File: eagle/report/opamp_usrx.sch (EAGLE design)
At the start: 11 parts, among them IC1 LM324N

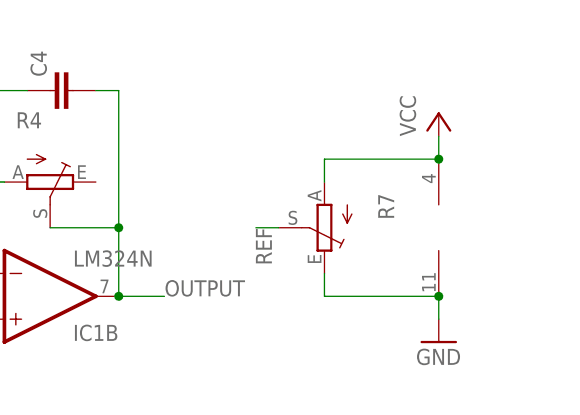
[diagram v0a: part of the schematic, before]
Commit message: Continued design and implementation.
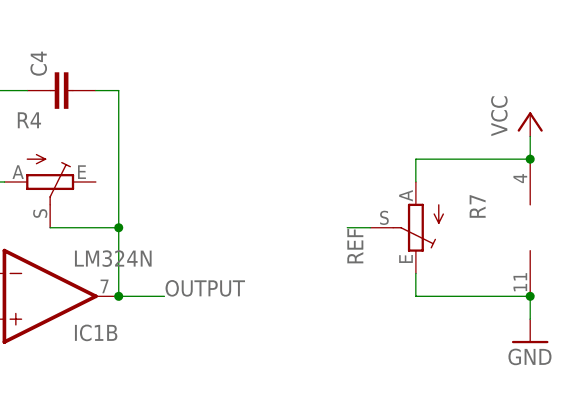
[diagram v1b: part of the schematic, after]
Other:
- moved on the sheet: R7
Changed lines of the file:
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@@
 <?xml version="1.0" encoding="utf-8"?>
 <!DOCTYPE eagle SYSTEM "eagle.dtd">
-<eagle version="6.3">
+<eagle version="6.4">
 <drawing>
 <settings>
@@
 <instance part="R3" gate="G$1" x="185.42" y="203.2"/>
 <instance part="R2" gate="1" x="160.02" y="215.9" rot="R270"/>
-<instance part="R7" gate="1" x="231.14" y="208.28" rot="R180"/>
+<instance part="R7" gate="1" x="241.3" y="208.28" rot="R180"/>
 <instance part="R4" gate="1" x="200.66" y="213.36" rot="R270"/>
 <instance part="C1" gate="G$1" x="132.08" y="205.74" rot="R90"/>
@@
 <instance part="C3" gate="G$1" x="172.72" y="203.2" rot="R90"/>
 <instance part="C4" gate="G$1" x="200.66" y="223.52" rot="R90"/>
-<instance part="IC1" gate="P" x="243.84" y="208.28"/>
-<instance part="GND2" gate="1" x="243.84" y="195.58"/>
+<instance part="IC1" gate="P" x="254" y="208.28"/>
+<instance part="GND2" gate="1" x="254" y="195.58"/>
 <instance part="U$2" gate="G$1" x="124.46" y="200.66" rot="R90"/>
 <instance part="GND7" gate="1" x="127" y="193.04"/>
-<instance part="P+1" gate="VCC" x="243.84" y="220.98"/>
+<instance part="P+1" gate="VCC" x="254" y="220.98"/>
 </instances>
 <busses>
@@
 <segment>
 <pinref part="R7" gate="1" pin="S"/>
-<wire x1="226.06" y1="208.28" x2="223.52" y2="208.28" width="0.1524" layer="91"/>
-<label x="223.52" y="208.28" size="1.778" layer="95" rot="R270"/>
+<wire x1="236.22" y1="208.28" x2="233.68" y2="208.28" width="0.1524" layer="91"/>
+<label x="233.68" y="208.28" size="1.778" layer="95" rot="R270"/>
 </segment>
 </net>
@@
 <segment>
 <pinref part="IC1" gate="P" pin="V-"/>
-<wire x1="243.84" y1="200.66" x2="231.14" y2="200.66" width="0.1524" layer="91"/>
+<wire x1="254" y1="200.66" x2="241.3" y2="200.66" width="0.1524" layer="91"/>
 <pinref part="R7" gate="1" pin="E"/>
-<wire x1="231.14" y1="200.66" x2="231.14" y2="203.2" width="0.1524" layer="91"/>
-<wire x1="243.84" y1="200.66" x2="243.84" y2="198.12" width="0.1524" layer="91"/>
-<junction x="243.84" y="200.66"/>
+<wire x1="241.3" y1="200.66" x2="241.3" y2="203.2" width="0.1524" layer="91"/>
+<wire x1="254" y1="200.66" x2="254" y2="198.12" width="0.1524" layer="91"/>
+<junction x="254" y="200.66"/>
 <pinref part="GND2" gate="1" pin="GND"/>
 </segment>
@@
 <pinref part="IC1" gate="P" pin="V+"/>
 <pinref part="P+1" gate="VCC" pin="VCC"/>
-<wire x1="243.84" y1="218.44" x2="243.84" y2="215.9" width="0.1524" layer="91"/>
+<wire x1="254" y1="218.44" x2="254" y2="215.9" width="0.1524" layer="91"/>
 <pinref part="R7" gate="1" pin="A"/>
-<wire x1="231.14" y1="215.9" x2="231.14" y2="213.36" width="0.1524" layer="91"/>
-<wire x1="231.14" y1="215.9" x2="243.84" y2="215.9" width="0.1524" layer="91"/>
-<junction x="243.84" y="215.9"/>
-</segment>
-</net>
+<wire x1="241.3" y1="215.9" x2="241.3" y2="213.36" width="0.1524" layer="91"/>
+<wire x1="241.3" y1="215.9" x2="254" y2="215.9" width="0.1524" layer="91"/>
+<junction x="254" y="215.9"/>
+</segment>
+</net>
